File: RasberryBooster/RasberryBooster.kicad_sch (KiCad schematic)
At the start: 14 parts, among them J1 Conn_01x02_Socket, J2 Capacitor, J3 Conn_01x02_Socket

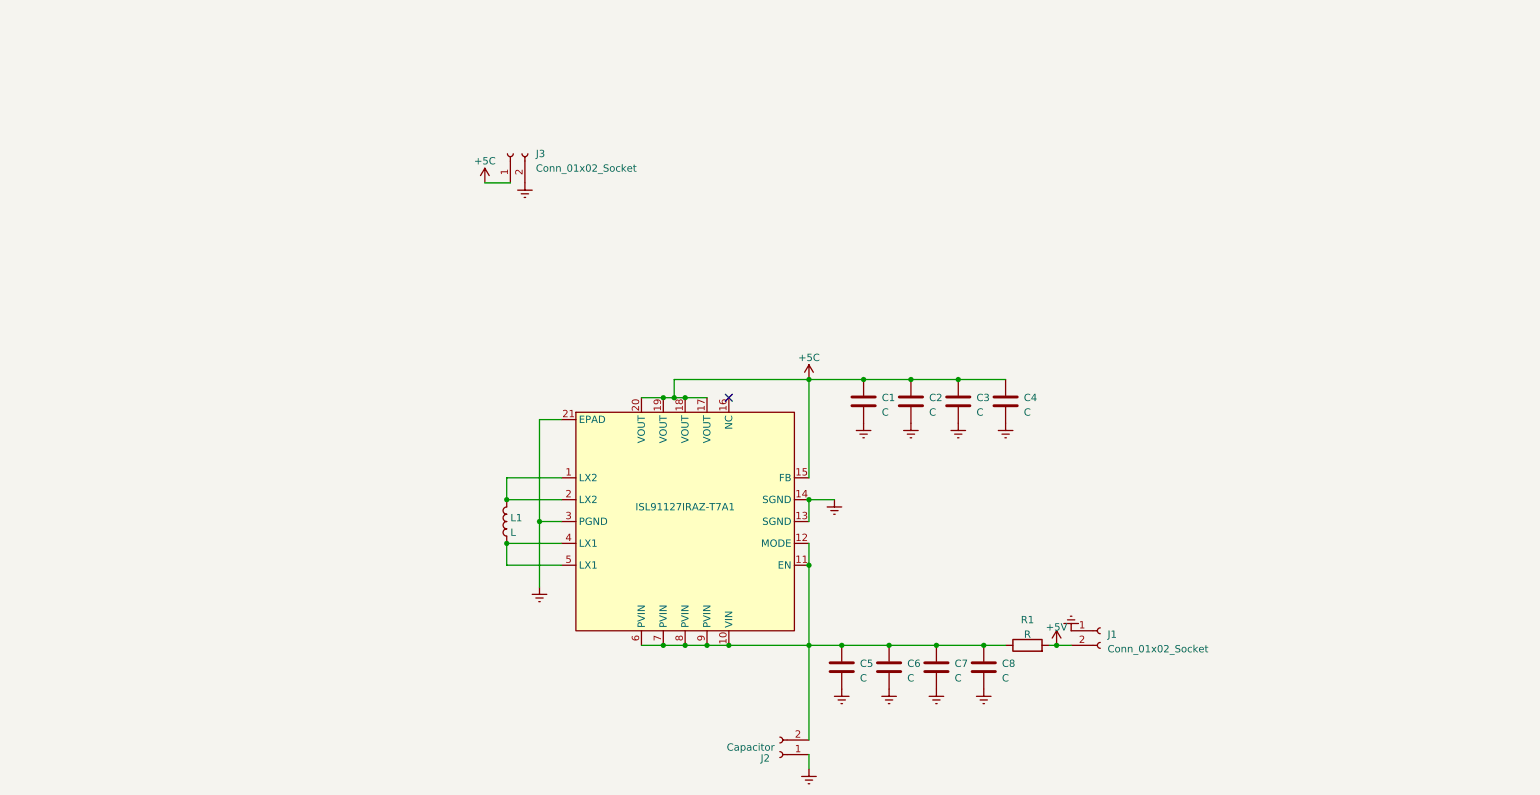
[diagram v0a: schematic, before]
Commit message: Finished PCB design
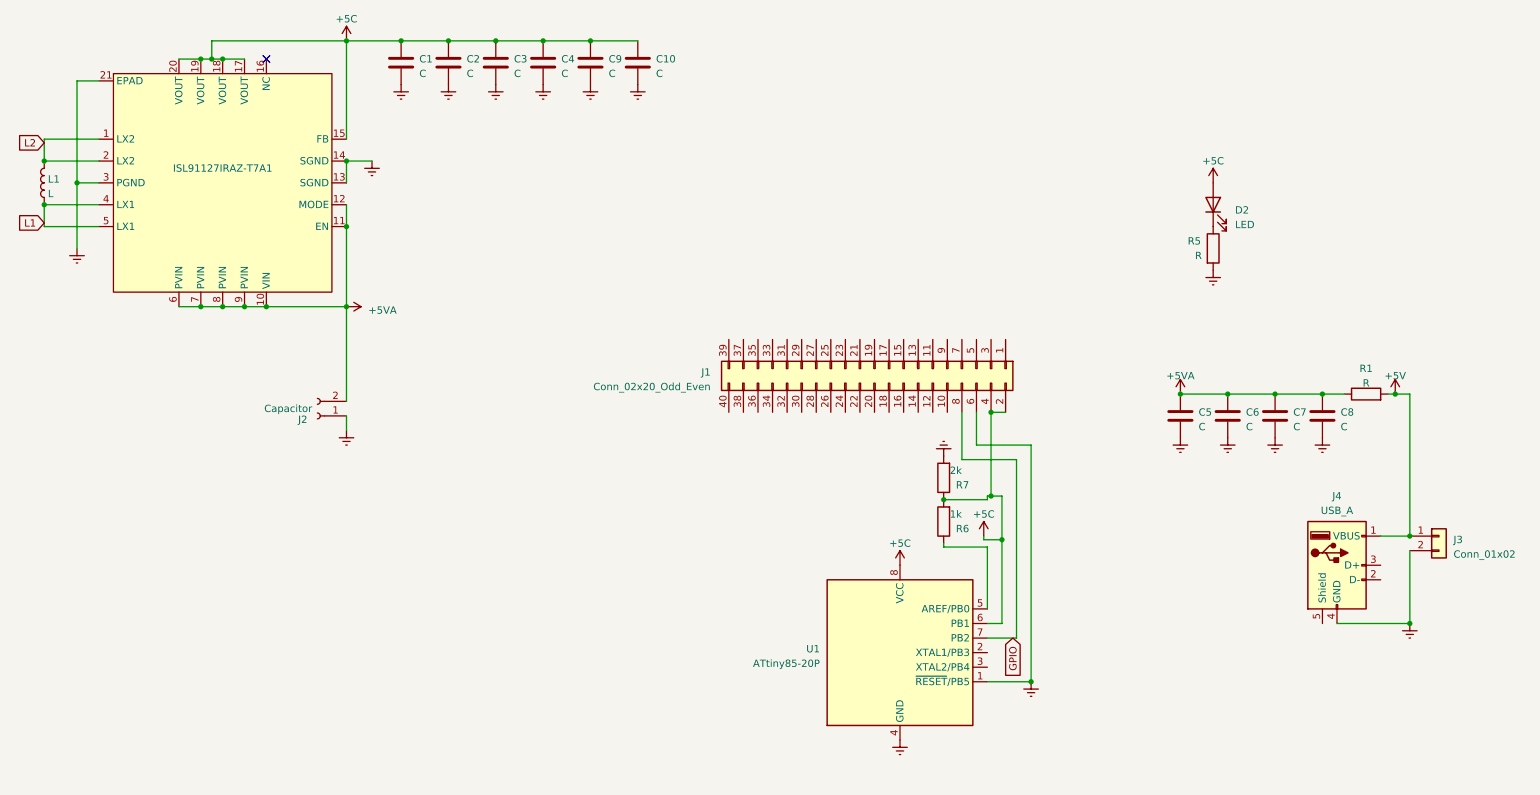
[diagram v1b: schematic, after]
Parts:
- removed J1, J3: Conn_01x02_Socket, Connector_PinHeader_2.54mm:PinHeader_1x02_P2.54mm_Horizontal, symbol Connector:Conn_01x02_Socket
- added C10, C9: C, Capacitor_SMD:C_0603_1608Metric, symbol Device:C
- added D2: LED, LED_SMD:LED_0603_1608Metric, symbol Device:LED
- added J1: Conn_02x20_Odd_Even, Connector_PinHeader_2.54mm:PinHeader_2x20_P2.54mm_Vertical, symbol Connector_Generic:Conn_02x20_Odd_Even
- added J3: Conn_01x02, Connector_PinSocket_2.54mm:PinSocket_1x02_P2.54mm_Vertical, symbol Connector_Generic:Conn_01x02
- added J4: USB_A, Connector_USB:USB_Micro-B_Molex-105017-0001, symbol Connector:USB_A
- added R5: R, Resistor_SMD:R_0603_1608Metric, symbol Device:R
- added R6: 1k, Resistor_SMD:R_0603_1608Metric, symbol Device:R
- added R7: 2k, Resistor_SMD:R_0603_1608Metric, symbol Device:R
- added U1: ATtiny85-20P, Package_DIP:DIP-8_W7.62mm, symbol MCU_Microchip_ATtiny:ATtiny85-20P
- J2: footprint Connector_JST:JST_ZE_B02B-ZESK-1D_1x02_P1.50mm_Vertical -> Connector_PinSocket_2.54mm:PinSocket_1x02_P2.54mm_Vertical
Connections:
- net +5C: now also C10.1, C9.1, D2.2 (A), J1.2 (Pin_2), J1.4 (Pin_4), R6.2, R7.1, U1.6 (PB1), U1.8 (VCC)
- net +5V: now also J3.1 (Pin_1), J4.1 (VBUS)
- net Earth: now also C10.2, C9.2, J1.6 (Pin_6), J3.2 (Pin_2), J4.4 (GND), R5.2, R7.2, U1.1 (~{RESET}/PB5), U1.4 (GND)
- net +5VA: now reaches C5.1, C6.1, C7.1, C8.1, ISL91127IRAZ-T7A1.10 (VIN), ISL91127IRAZ-T7A1.11 (EN), ISL91127IRAZ-T7A1.12 (MODE), ISL91127IRAZ-T7A1.6 (PVIN), ISL91127IRAZ-T7A1.7 (PVIN), ISL91127IRAZ-T7A1.8 (PVIN), ISL91127IRAZ-T7A1.9 (PVIN), J2.2 (Pin_2), R1.1
- net L1: now reaches ISL91127IRAZ-T7A1.4 (LX1), ISL91127IRAZ-T7A1.5 (LX1), L1.1
- net L2: now reaches ISL91127IRAZ-T7A1.1 (LX2), ISL91127IRAZ-T7A1.2 (LX2), L1.2
- new net: R6.1, U1.5 (AREF/PB0)
- new net: D2.1 (K), R5.1
- new net GPIO: J1.8 (Pin_8), U1.7 (PB2)
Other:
- moved on the sheet: C1, C2, C3, C4, C5, C6, C7, C8, ISL91127IRAZ-T7A1, J2, L1, R1
